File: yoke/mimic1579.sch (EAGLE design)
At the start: 75 parts, among them P1 44PINEDGE, P2 2K, P3 2K, Q1 2N3904, Q13 2N3904, Q14 2N3904, Q15 2N3906, Q16 2N3904, Q2 2N3906, Q3 2N3906, Q4 2N3906, Q5 2N3904, Q6 2N3904, Q7 2N3906, Q8 2N3904, Q9 2N3904

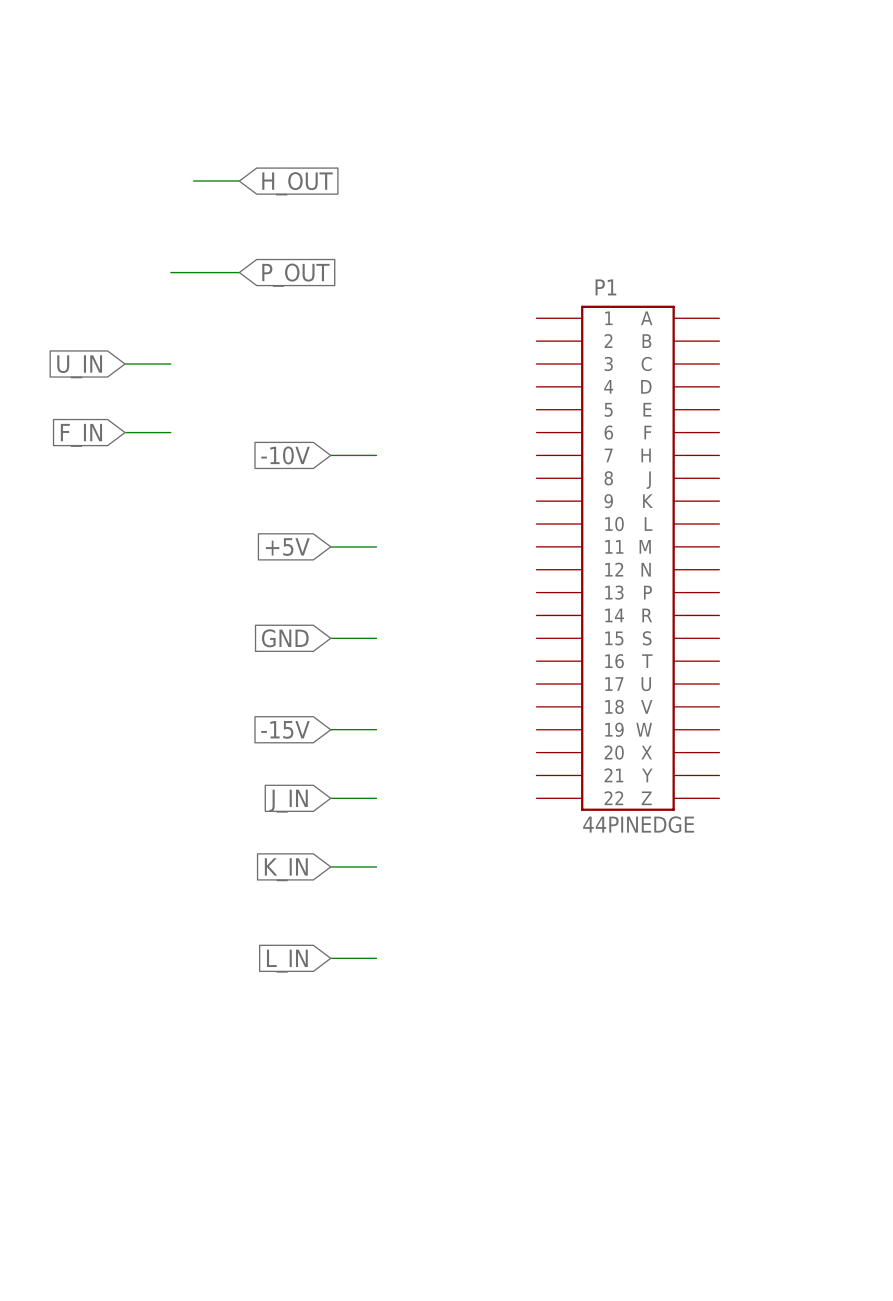
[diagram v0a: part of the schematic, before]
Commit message: update netlist
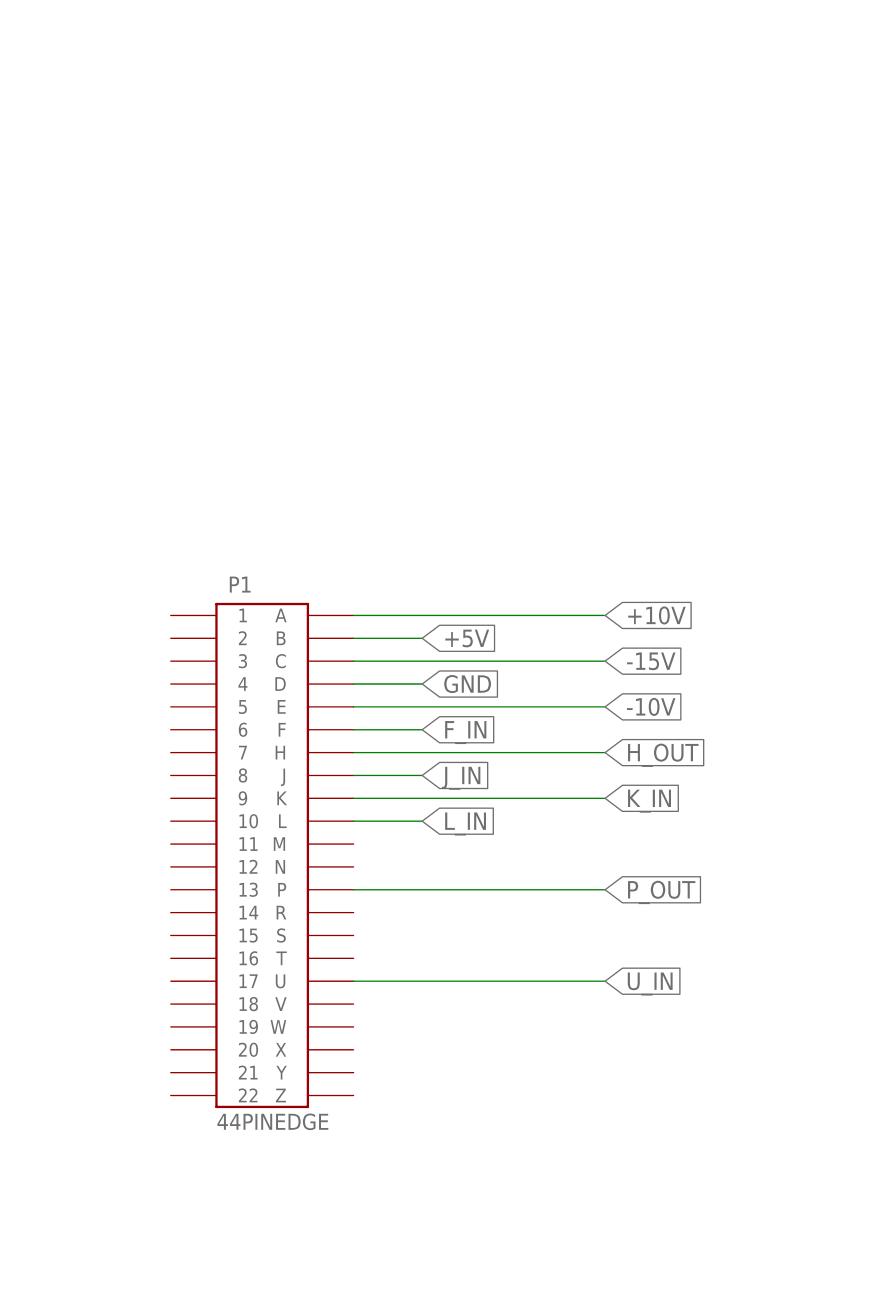
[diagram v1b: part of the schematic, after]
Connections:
- new net +10V: P1.A
- new net +5V: P1.B
- net -10V: now also P1.E
- net -15V: now also P1.C
- net F_IN: now also P1.F
- net GND: now also P1.D
- net H_OUT: now also P1.H
- net J_IN: now also P1.J
- net K_IN: now also P1.K
- net L_IN: now also P1.L
- net P_OUT: now also P1.P
- net U_IN: now also P1.U
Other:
- moved on the sheet: P1
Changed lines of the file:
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@@
 </classes>
 <parts>
-<part name="P1" library="keiths" deviceset="44PINEDGE" device=""/>
 <part name="Q5" library="keiths" deviceset="2N3904" device=""/>
 <part name="R2" library="keiths" deviceset="R-1/4WATT" device="" value="4.7K"/>
@@
 <part name="SUPPLY19" library="keiths" deviceset="+5V" device=""/>
 <part name="FRAME1" library="frames" deviceset="FRAME_C_L" device=""/>
+<part name="P1" library="keiths" deviceset="44PINEDGE" device=""/>
 </parts>
 <sheets>
@@
 </plain>
 <instances>
-<instance part="P1" gate="G$1" x="134.62" y="220.98"/>
 <instance part="Q5" gate="G1" x="330.2" y="332.74"/>
 <instance part="R2" gate="&gt;NAME" x="322.58" y="342.9" smashed="yes" rot="MR90">
@@
 <instance part="FRAME1" gate="G$1" x="0" y="0"/>
 <instance part="FRAME1" gate="G$2" x="452.12" y="0"/>
+<instance part="P1" gate="G$1" x="93.98" y="187.96"/>
 </instances>
 <busses>
@@
 </segment>
 <segment>
-<label x="78.74" y="233.68" size="1.9304" layer="95" rot="R180" xref="yes"/>
-<wire x1="83.82" y1="233.68" x2="78.74" y2="233.68" width="0.1524" layer="91"/>
+<label x="111.76" y="200.66" size="1.9304" layer="95" font="vector" ratio="10" xref="yes"/>
+<pinref part="P1" gate="G$1" pin="F"/>
+<wire x1="104.14" y1="200.66" x2="111.76" y2="200.66" width="0.1524" layer="91"/>
 </segment>
 </net>
@@
 </segment>
 <segment>
-<wire x1="106.68" y1="210.82" x2="101.6" y2="210.82" width="0.1524" layer="91"/>
-<label x="101.6" y="210.82" size="1.9304" layer="95" font="vector" ratio="10" rot="MR0" xref="yes"/>
+<pinref part="P1" gate="G$1" pin="D"/>
+<wire x1="104.14" y1="205.74" x2="111.76" y2="205.74" width="0.1524" layer="91"/>
+<label x="111.76" y="205.74" size="1.9304" layer="95" font="vector" ratio="10" xref="yes"/>
 </segment>
 </net>
@@
 </segment>
 <segment>
-<wire x1="83.82" y1="251.46" x2="91.44" y2="251.46" width="0.1524" layer="91"/>
-<label x="91.44" y="251.46" size="1.9304" layer="95" font="vector" ratio="10" xref="yes"/>
+<wire x1="104.14" y1="182.88" x2="132.08" y2="182.88" width="0.1524" layer="91"/>
+<label x="132.08" y="182.88" size="1.9304" layer="95" font="vector" ratio="10" xref="yes"/>
+<pinref part="P1" gate="G$1" pin="P"/>
 </segment>
 </net>
@@
 </segment>
 <segment>
-<wire x1="91.44" y1="261.62" x2="86.36" y2="261.62" width="0.1524" layer="91"/>
-<label x="91.44" y="261.62" size="1.9304" layer="95" font="vector" ratio="10" xref="yes"/>
+<label x="132.08" y="198.12" size="1.9304" layer="95" font="vector" ratio="10" xref="yes"/>
+<pinref part="P1" gate="G$1" pin="H"/>
+<wire x1="104.14" y1="198.12" x2="132.08" y2="198.12" width="0.1524" layer="91"/>
 </segment>
 </net>
@@
 </segment>
 <segment>
-<label x="101.6" y="231.14" size="1.9304" layer="95" font="vector" ratio="10" rot="MR0" xref="yes"/>
-<wire x1="106.68" y1="231.14" x2="101.6" y2="231.14" width="0.1524" layer="91"/>
+<label x="132.08" y="203.2" size="1.9304" layer="95" font="vector" ratio="10" rot="MR180" xref="yes"/>
+<pinref part="P1" gate="G$1" pin="E"/>
+<wire x1="104.14" y1="203.2" x2="132.08" y2="203.2" width="0.1524" layer="91"/>
 </segment>
 </net>
@@
 </segment>
 <segment>
-<label x="101.6" y="193.04" size="1.9304" layer="95" font="vector" ratio="10" rot="MR0" xref="yes"/>
-<wire x1="101.6" y1="193.04" x2="106.68" y2="193.04" width="0.1524" layer="91"/>
+<label x="111.76" y="195.58" size="1.9304" layer="95" font="vector" ratio="10" rot="MR180" xref="yes"/>
+<wire x1="111.76" y1="195.58" x2="104.14" y2="195.58" width="0.1524" layer="91"/>
+<pinref part="P1" gate="G$1" pin="J"/>
 </segment>
 </net>
@@
 </segment>
 <segment>
-<label x="101.6" y="175.26" size="1.9304" layer="95" font="vector" ratio="10" rot="MR0" xref="yes"/>
-<wire x1="101.6" y1="175.26" x2="106.68" y2="175.26" width="0.1524" layer="91"/>
+<label x="111.76" y="190.5" size="1.9304" layer="95" font="vector" ratio="10" rot="MR180" xref="yes"/>
+<wire x1="111.76" y1="190.5" x2="104.14" y2="190.5" width="0.1524" layer="91"/>
+<pinref part="P1" gate="G$1" pin="L"/>
 </segment>
 </net>
@@
 </segment>
 <segment>
-<label x="78.74" y="241.3" size="1.9304" layer="95" rot="MR0" xref="yes"/>
-<wire x1="83.82" y1="241.3" x2="78.74" y2="241.3" width="0.1524" layer="91"/>
+<label x="132.08" y="172.72" size="1.9304" layer="95" font="vector" ratio="10" rot="MR180" xref="yes"/>
+<wire x1="104.14" y1="172.72" x2="132.08" y2="172.72" width="0.1524" layer="91"/>
+<pinref part="P1" gate="G$1" pin="U"/>
 </segment>
 </net>
@@
 </segment>
 <segment>
-<label x="101.6" y="200.66" size="1.9304" layer="95" font="vector" ratio="10" rot="MR0" xref="yes"/>
-<wire x1="106.68" y1="200.66" x2="101.6" y2="200.66" width="0.1524" layer="91"/>
+<pinref part="P1" gate="G$1" pin="C"/>
+<wire x1="104.14" y1="208.28" x2="132.08" y2="208.28" width="0.1524" layer="91"/>
+<label x="132.08" y="208.28" size="1.9304" layer="95" font="vector" ratio="10" xref="yes"/>
 </segment>
 </net>
@@
 </segment>
 <segment>
-<wire x1="101.6" y1="185.42" x2="106.68" y2="185.42" width="0.1524" layer="91"/>
-<label x="101.6" y="185.42" size="1.9304" layer="95" font="vector" ratio="10" rot="MR0" xref="yes"/>
+<wire x1="132.08" y1="193.04" x2="104.14" y2="193.04" width="0.1524" layer="91"/>
+<label x="132.08" y="193.04" size="1.9304" layer="95" font="vector" ratio="10" rot="MR180" xref="yes"/>
+<pinref part="P1" gate="G$1" pin="K"/>
 </segment>
 </net>
@@
 </segment>
 <segment>
-<wire x1="106.68" y1="220.98" x2="101.6" y2="220.98" width="0.1524" layer="91"/>
-<label x="101.6" y="220.98" size="1.9304" layer="95" rot="R180" xref="yes"/>
-</segment>
-</net>
+<label x="111.76" y="210.82" size="1.9304" layer="95" font="vector" ratio="10" xref="yes"/>
+<pinref part="P1" gate="G$1" pin="B"/>
+<wire x1="104.14" y1="210.82" x2="111.76" y2="210.82" width="0.1524" layer="91"/>
+</segment>
+</net>
+<net name="+10V" class="0">
+<segment>
+<pinref part="P1" gate="G$1" pin="A"/>
+<wire x1="104.14" y1="213.36" x2="132.08" y2="213.36" width="0.1524" layer="91"/>
+<label x="132.08" y="213.36" size="1.9304" layer="95" font="vector" ratio="10" xref="yes"/>
+</segment>
+</net>
